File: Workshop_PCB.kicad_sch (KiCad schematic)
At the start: 15 parts, among them J1 Conn_01x04, SW1 SW_MEC_5E, U1 STM32F042C6Tx, U2 AMS1117-3.3

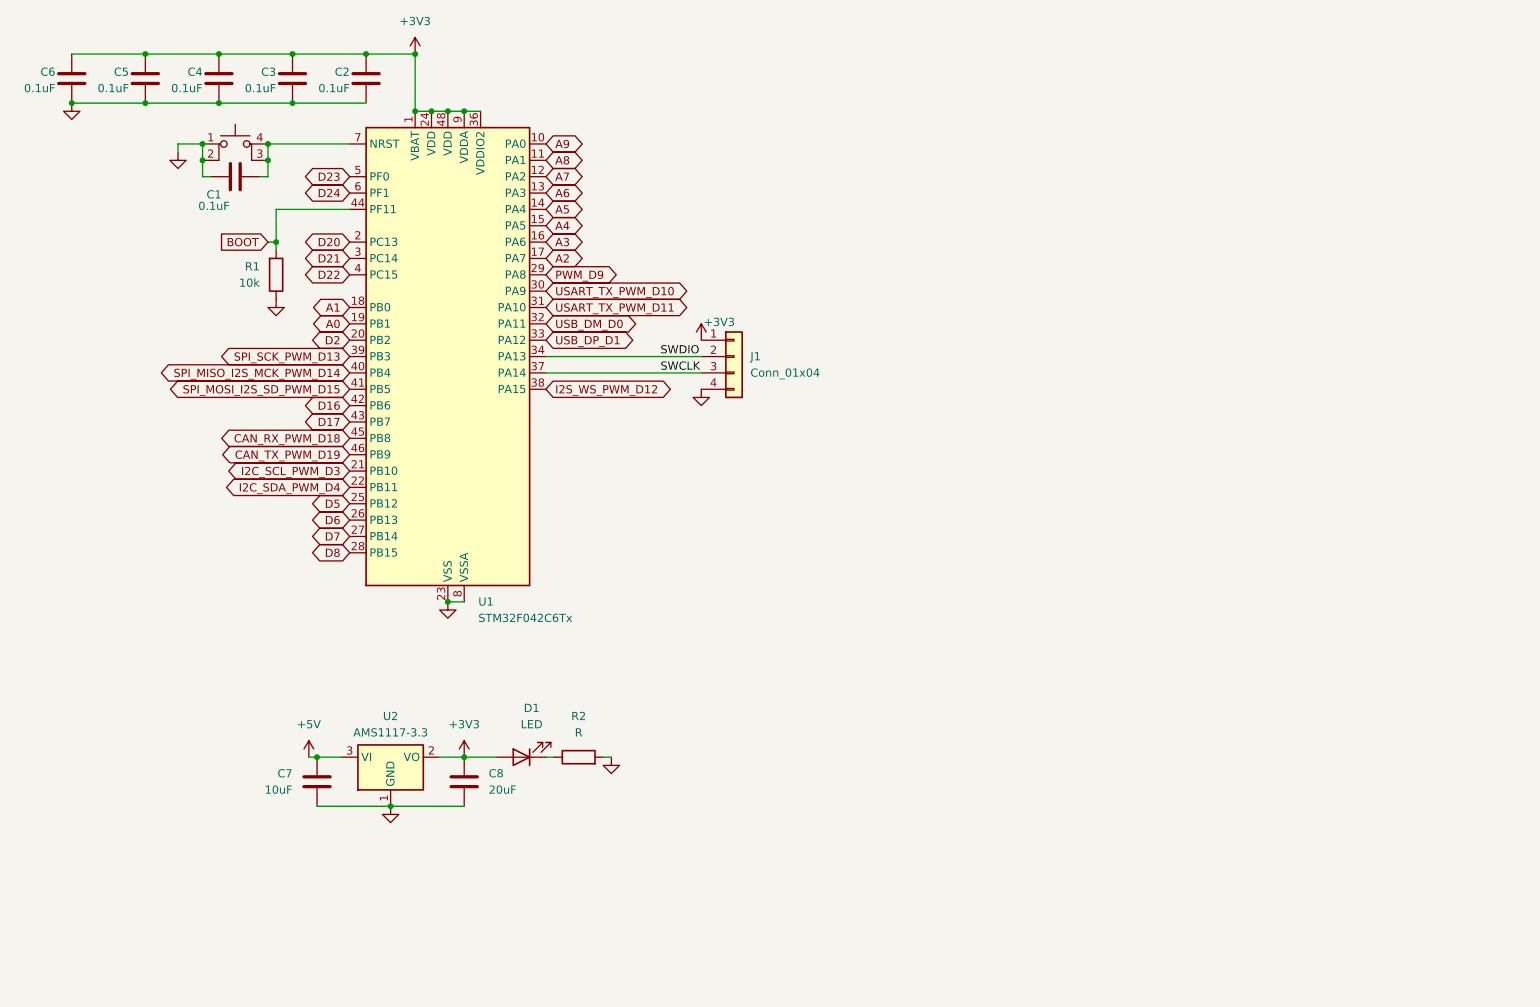
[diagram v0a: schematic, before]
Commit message: Finish schematic, assign components and footprints
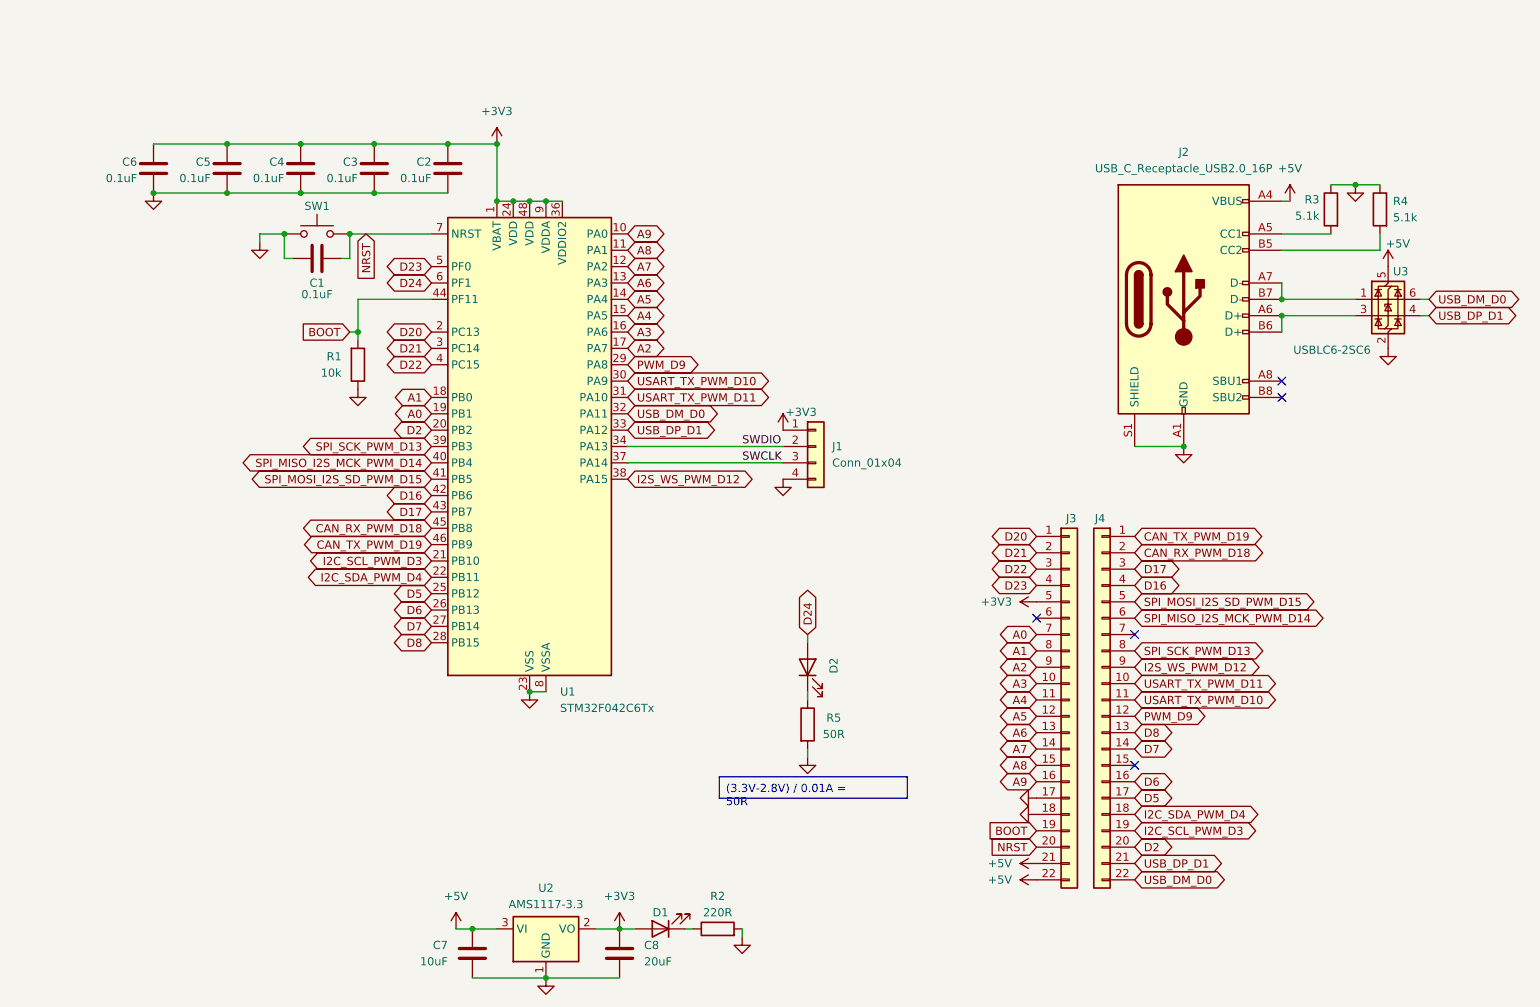
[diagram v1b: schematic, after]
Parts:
- removed SW1: SW_MEC_5E, symbol Switch:SW_MEC_5E
- added D2: LED, LED_SMD:LED_0805_2012Metric, symbol Device:LED
- added J2: USB_C_Receptacle_USB2.0_16P, Connector_USB:USB_C_Receptacle_GCT_USB4105-xx-A_16P_TopMnt_Horizontal, symbol Connector:USB_C_Receptacle_USB2.0_16P
- added J3, J4: Conn_01x22, Connector_PinSocket_2.54mm:PinSocket_1x22_P2.54mm_Vertical, symbol Connector_Generic:Conn_01x22
- added R3, R4: 5.1k, Resistor_SMD:R_0603_1608Metric, symbol Device:R
- added R5: 50R, Resistor_SMD:R_0603_1608Metric, symbol Device:R
- added SW1: SW_Push, Button_Switch_SMD:SW_Push_1P1T_XKB_TS-1187A, symbol Switch:SW_Push
- added U3: USBLC6-2SC6, Package_TO_SOT_SMD:SOT-23-6, symbol Power_Protection:USBLC6-2SC6
- C1, C2, C3, C4, C5, C6, C7, C8: footprint (none) -> Capacitor_SMD:C_0603_1608Metric
- D1: footprint (none) -> LED_SMD:LED_0805_2012Metric; LCSC (none) -> C2297
- J1: footprint (none) -> Connector_PinSocket_2.54mm:PinSocket_1x04_P2.54mm_Horizontal
- R1: footprint (none) -> Resistor_SMD:R_0603_1608Metric
- R2: value R -> 220R; footprint (none) -> Resistor_SMD:R_0603_1608Metric
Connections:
- net +3V3: now also J3.5 (Pin_5)
- net +5V: now also J2.A4 (VBUS), J2.A9 (VBUS), J2.B4 (VBUS), J2.B9 (VBUS), J3.21 (Pin_21), J3.22 (Pin_22), U3.5 (VBUS)
- net A0: now also J3.7 (Pin_7)
- net A1: now also J3.8 (Pin_8)
- net A2: now also J3.9 (Pin_9)
- net A3: now also J3.10 (Pin_10)
- net A4: now also J3.11 (Pin_11)
- net A5: now also J3.12 (Pin_12)
- net A6: now also J3.13 (Pin_13)
- net A7: now also J3.14 (Pin_14)
- net A8: now also J3.15 (Pin_15)
- net A9: now also J3.16 (Pin_16)
- net BOOT: now also J3.19 (Pin_19)
- net CAN_RX_PWM_D18: now also J4.2 (Pin_2)
- net CAN_TX_PWM_D19: now also J4.1 (Pin_1)
- net D16: now also J4.4 (Pin_4)
- net D17: now also J4.3 (Pin_3)
- net D2: now also J4.20 (Pin_20)
- net D20: now also J3.1 (Pin_1)
- net D21: now also J3.2 (Pin_2)
- net D22: now also J3.3 (Pin_3)
- net D23: now also J3.4 (Pin_4)
- net D24: now also D2.2 (A)
- net D5: now also J4.17 (Pin_17)
- net D6: now also J4.16 (Pin_16)
- net D7: now also J4.14 (Pin_14)
- net D8: now also J4.13 (Pin_13)
- net GND: now also J2.A1 (GND), J2.A12 (GND), J2.B1 (GND), J2.B12 (GND), J2.S1 (SHIELD), J3.17 (Pin_17), J3.18 (Pin_18), R3.1, R4.1, R5.2, SW1.1, U3.2 (GND)
- net I2C_SCL_PWM_D3: now also J4.19 (Pin_19)
- net I2C_SDA_PWM_D4: now also J4.18 (Pin_18)
- net I2S_WS_PWM_D12: now also J4.9 (Pin_9)
- net PWM_D9: now also J4.12 (Pin_12)
- net SPI_MISO_I2S_MCK_PWM_D14: now also J4.6 (Pin_6)
- net SPI_MOSI_I2S_SD_PWM_D15: now also J4.5 (Pin_5)
- net SPI_SCK_PWM_D13: now also J4.8 (Pin_8)
- net USART_TX_PWM_D10: now also J4.11 (Pin_11)
- net USART_TX_PWM_D11: now also J4.10 (Pin_10)
- net USB_DM_D0: now also J4.22 (Pin_22), U3.6 (I/O1)
- net USB_DP_D1: now also J4.21 (Pin_21), U3.4 (I/O2)
- net NRST: now reaches C1.2, U1.7 (NRST)
- net NRST: now also J3.20 (Pin_20), SW1.2
- new net: D2.1 (K), R5.1
- new net: J2.B5 (CC2), R4.2
- new net: J2.A5 (CC1), R3.2
- new net: J2.A6 (D+), J2.B6 (D+), U3.3 (I/O2)
- new net: J2.A7 (D-), J2.B7 (D-), U3.1 (I/O1)
- no-connect marks 0 -> 5
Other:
- title: (none) -> Hackpill
- moved on the sheet: C1, C2, C3, C4, C5, C6, C7, C8, J1, R1, U1, U2
